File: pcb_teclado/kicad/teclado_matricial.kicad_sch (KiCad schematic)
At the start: 1 part, among them SW2 PushButton 6mm 4pin

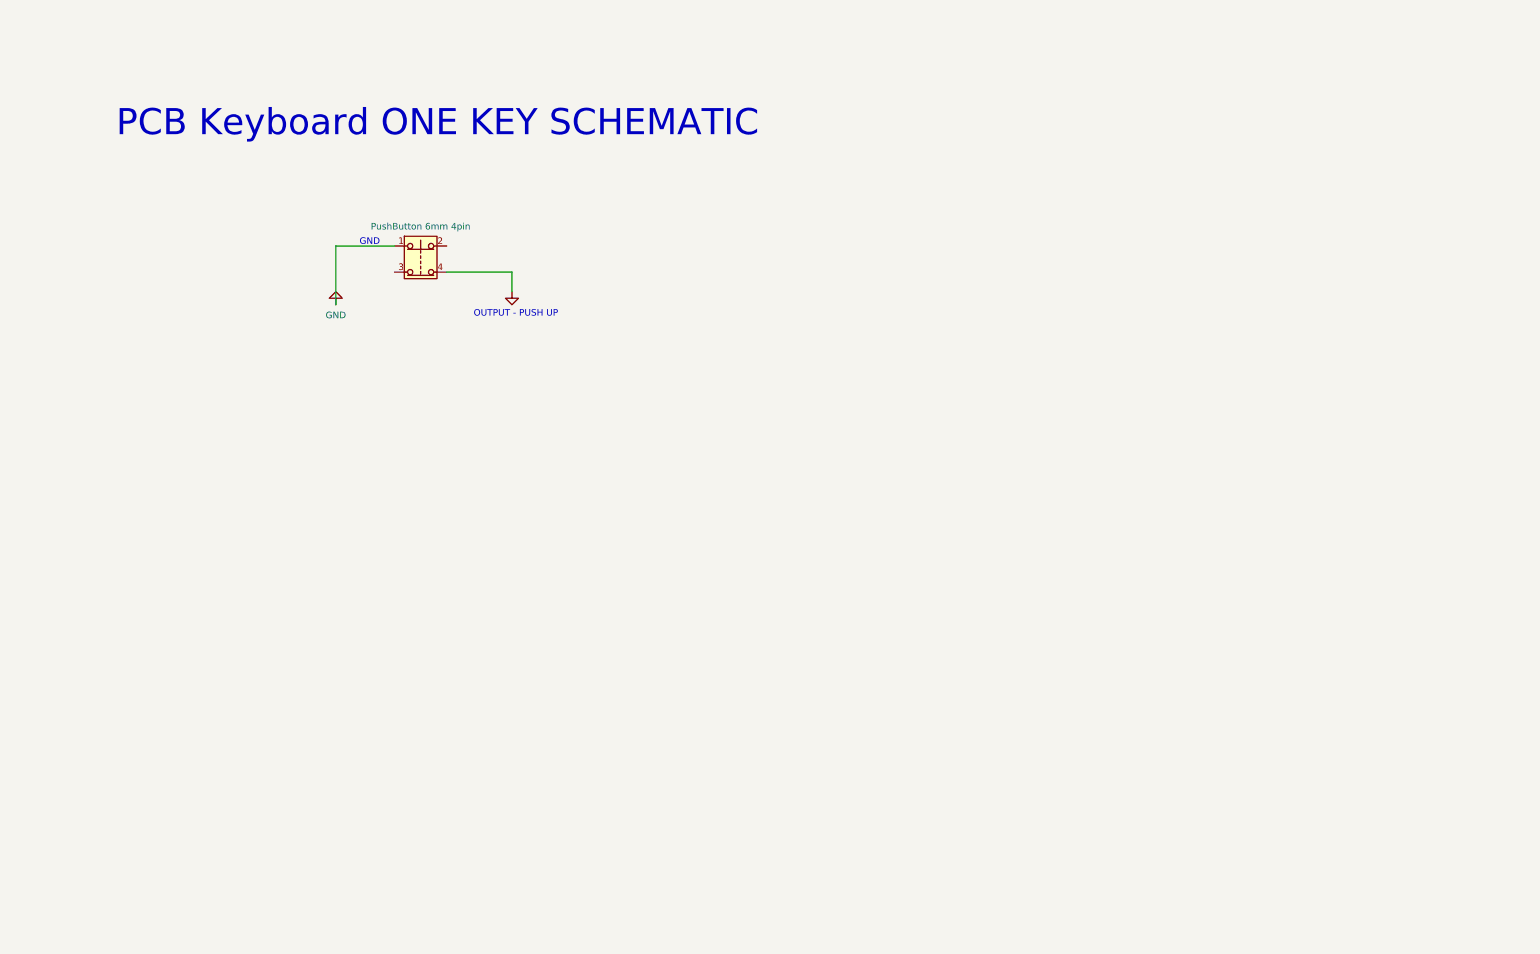
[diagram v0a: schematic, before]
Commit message: Updated cart and schematics
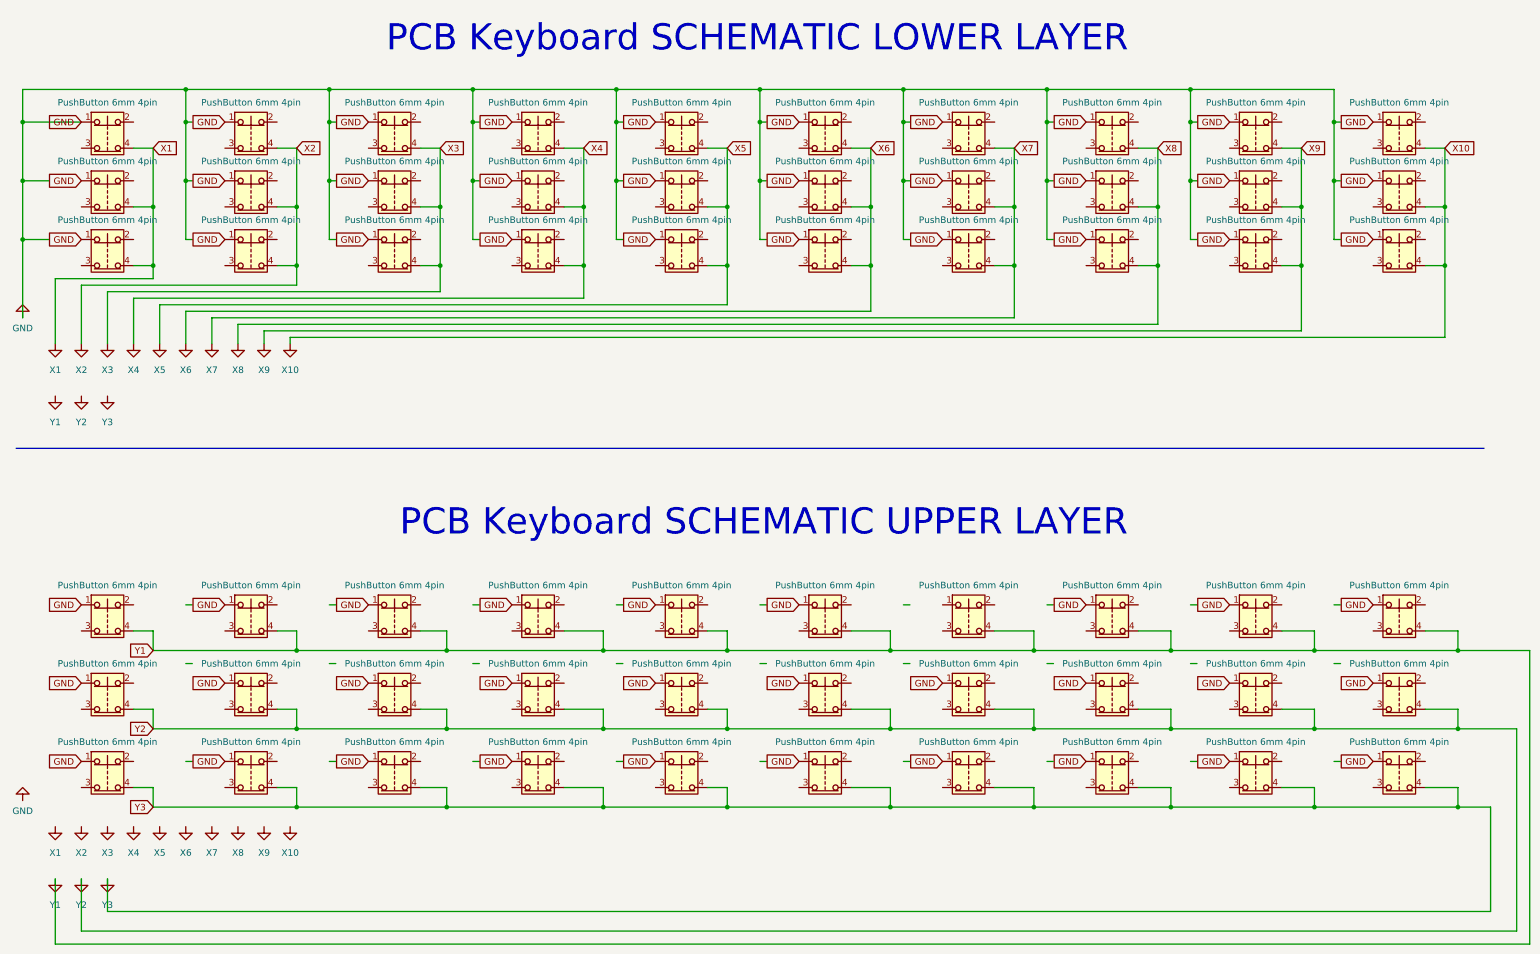
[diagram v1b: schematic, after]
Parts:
- added SW1, SW10, SW11, SW12, SW13, SW14, SW15, SW16, SW17, SW18, SW19, SW20, SW21, SW22, SW23, SW24, SW25, SW26, SW27, SW28, SW29, SW3, SW30, SW31, SW32, SW33, SW34, SW35, SW36, SW37, SW38, SW39, SW4, SW40, SW41, SW42, SW43, SW44, SW45, SW46, SW47, SW48, SW49, SW5, SW50, SW51, SW52, SW53, SW54, SW55, SW56, SW57, SW58, SW59, SW6, SW60, SW7, SW8, SW9: PushButton 6mm 4pin, symbol Switch:SW_Push_Open_Dual
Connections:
- net GND: now also SW1.1, SW10.1, SW11.1, SW12.1, SW13.1, SW14.1, SW15.1, SW16.1, SW17.1, SW18.1, SW19.1, SW20.1, SW21.1, SW22.1, SW23.1, SW24.1, SW25.1, SW26.1, SW27.1, SW28.1, SW29.1, SW3.1, SW30.1, SW31.1, SW32.1, SW33.1, SW34.1, SW35.1, SW36.1, SW37.1, SW38.1, SW39.1, SW4.1, SW40.1, SW41.1, SW42.1, SW43.1, SW44.1, SW45.1, SW46.1, SW47.1, SW48.1, SW5.1, SW50.1, SW51.1, SW52.1, SW53.1, SW54.1, SW55.1, SW56.1, SW57.1, SW58.1, SW59.1, SW6.1, SW60.1, SW7.1, SW8.1, SW9.1; no longer SW2.4
- new net X1: SW1.4, SW2.4, SW3.4
- new net X10: SW28.4, SW29.4, SW30.4
- new net X2: SW4.4, SW5.4, SW6.4
- new net X3: SW7.4, SW8.4, SW9.4
- new net X4: SW10.4, SW11.4, SW12.4
- new net X5: SW13.4, SW14.4, SW15.4
- new net X6: SW16.4, SW17.4, SW18.4
- new net X7: SW19.4, SW20.4, SW21.4
- new net X8: SW22.4, SW23.4, SW24.4
- new net X9: SW25.4, SW26.4, SW27.4
- new net Y1: SW31.4, SW34.4, SW37.4, SW40.4, SW43.4, SW46.4, SW49.4, SW52.4, SW55.4, SW58.4
- new net Y2: SW32.4, SW35.4, SW38.4, SW41.4, SW44.4, SW47.4, SW50.4, SW53.4, SW56.4, SW59.4
- new net Y3: SW33.4, SW36.4, SW39.4, SW42.4, SW45.4, SW48.4, SW51.4, SW54.4, SW57.4, SW60.4
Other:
- note added: "PCB Keyboard SCHEMATIC LOWER LAYER"
- note added: "PCB Keyboard SCHEMATIC UPPER LAYER"
- note removed: "GND"
- note removed: "OUTPUT - PUSH UP"
- note removed: "PCB Keyboard ONE KEY SCHEMATIC"
